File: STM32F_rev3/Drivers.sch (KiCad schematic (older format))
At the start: 28 parts, among them Q1 ISL9V5045S3ST, Q2 ISL9V5045S3ST, Q3 ISL9V5045S3ST, Q4 ISL9V5045S3ST

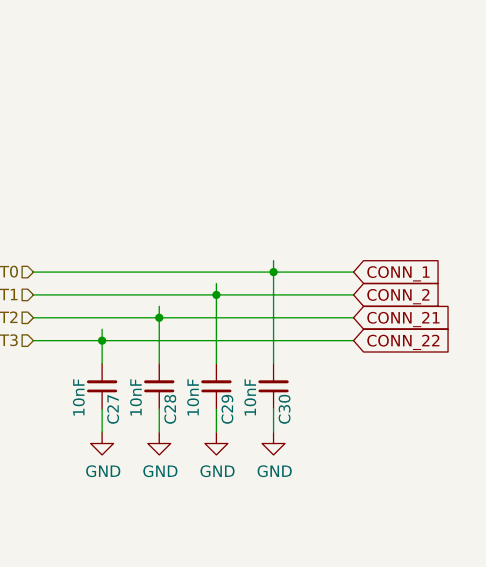
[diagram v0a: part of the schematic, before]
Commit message: WIP V3
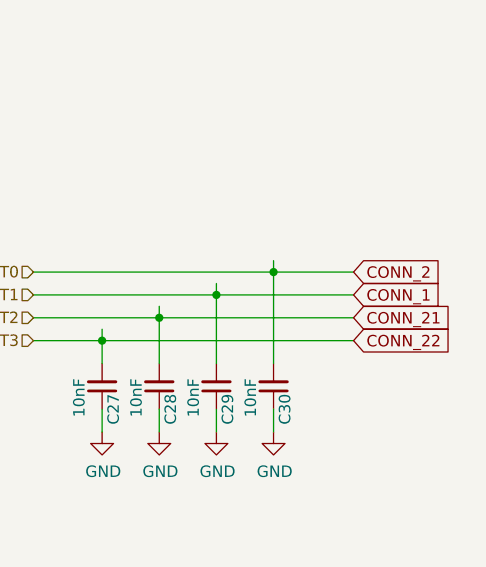
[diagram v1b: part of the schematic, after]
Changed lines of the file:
@@
 	4050 3200 4050 4250
 Connection ~ 4050 4250
+Text GLabel 6500 5900 2    50   Input ~ 0
+CONN_1
 Text GLabel 6500 5800 2    50   Input ~ 0
-CONN_1
-Text GLabel 6500 5900 2    50   Input ~ 0
 CONN_2
 Text GLabel 6500 6000 2    50   Input ~ 0
